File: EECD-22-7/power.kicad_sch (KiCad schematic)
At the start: 16 parts, among them U3 LMR54406DBVR, U4 LMR54406DBVR

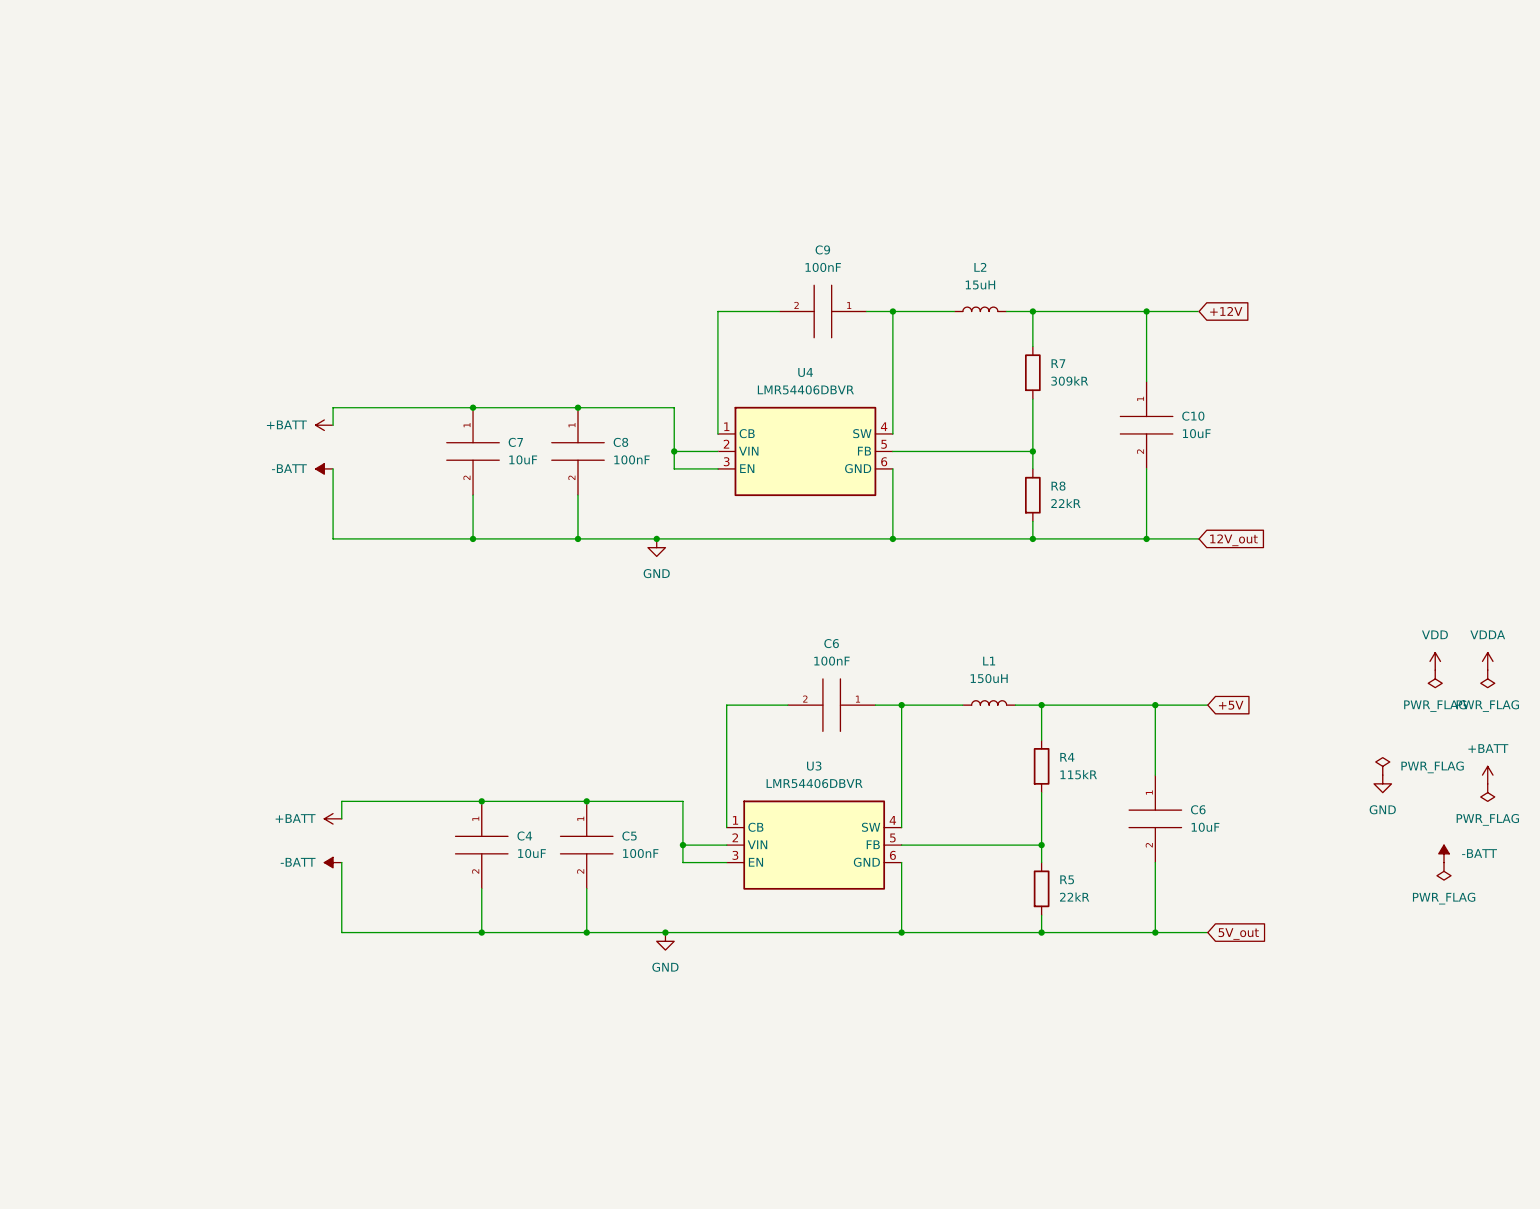
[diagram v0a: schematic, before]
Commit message: Add files via upload
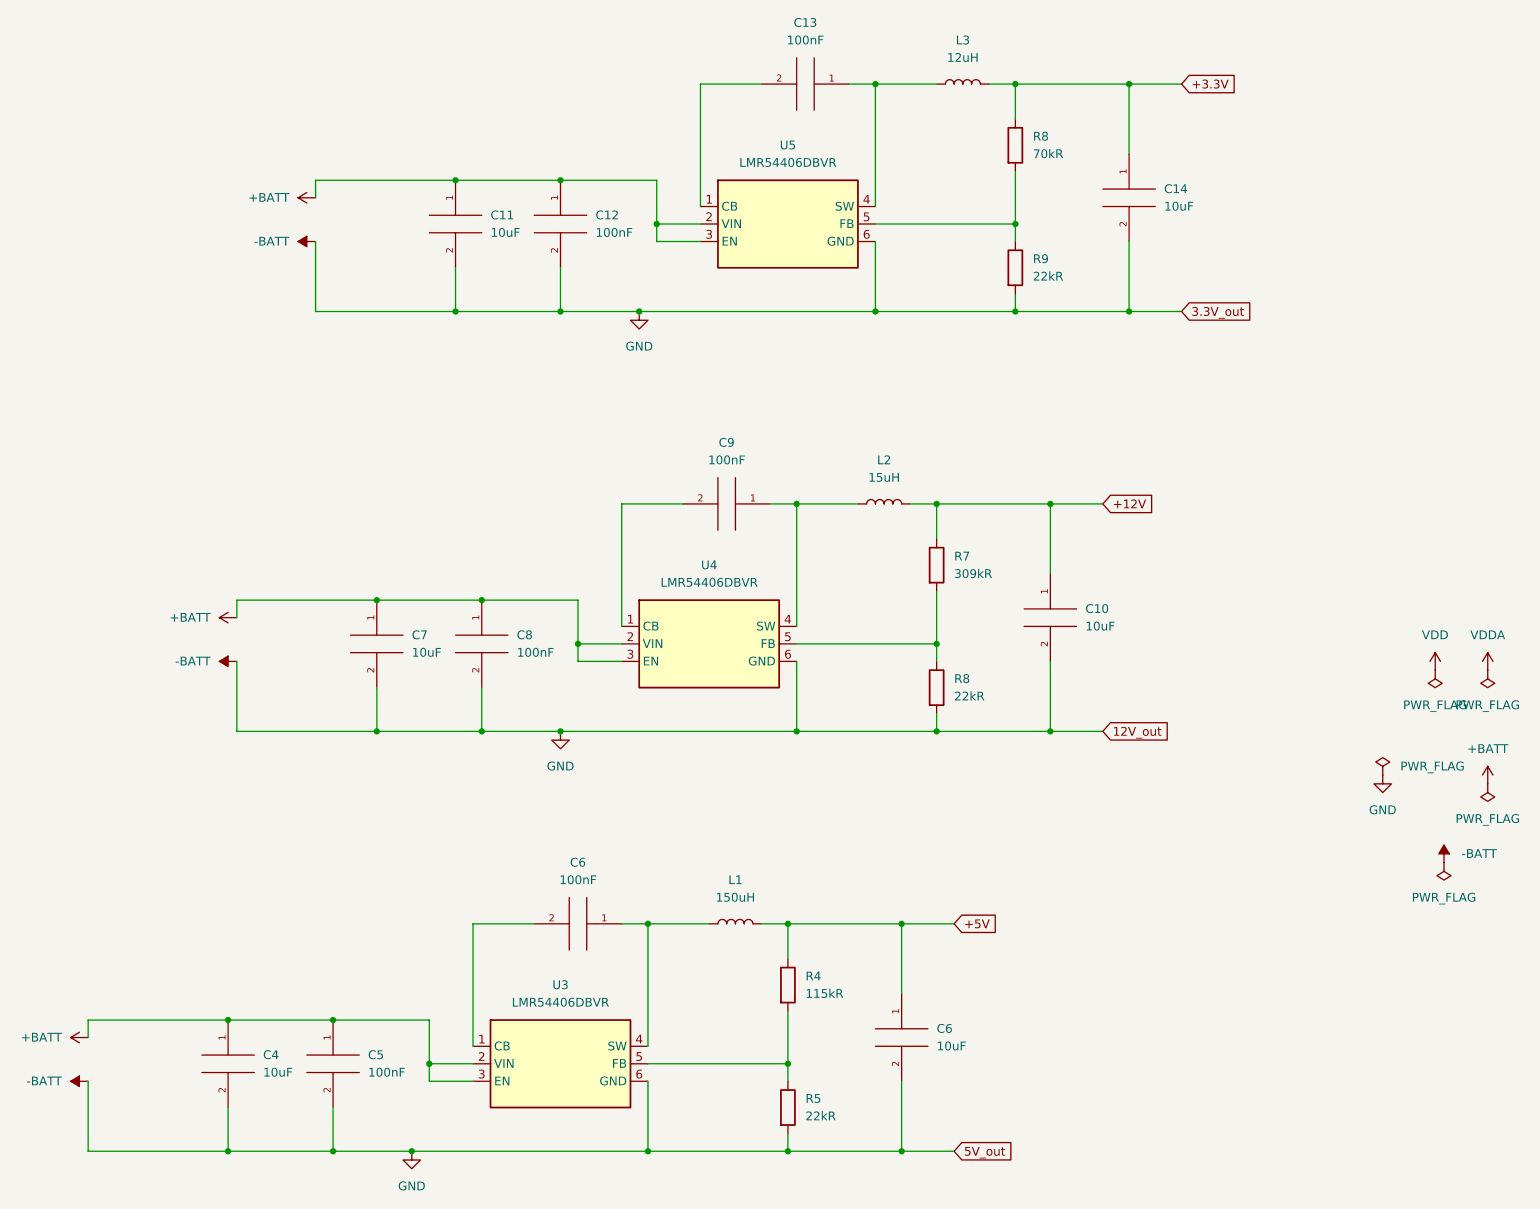
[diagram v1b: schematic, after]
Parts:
- added C11, C14: 10uF, symbol pspice:C
- added C12, C13: 100nF, symbol pspice:C
- added L3: 12uH, symbol Device:L
- added R8: 70kR, symbol Device:R
- added R9: 22kR, symbol Device:R
- added U5: LMR54406DBVR, symbol Regulator_Switching:LM5181NGUR
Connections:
- net +BATT: now also C11.1, C12.1, U5.2 (VIN), U5.3 (EN)
- net -BATT: now also C11.2, C12.2, C14.2, R9.2, U5.6 (GND)
- new net: R8.2, R9.1, U5.5 (FB)
- new net: C13.1, L3.1, U5.4 (SW)
- new net: C13.2, U5.1 (CB)
- new net +3.3V: C14.1, L3.2, R8.1
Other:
- moved on the sheet: C10, C4, C5, C6, C7, C8, C9, L1, L2, R4, R5, R7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
